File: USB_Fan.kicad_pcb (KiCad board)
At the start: 4 copper layers, 35.1 x 24.9 mm, 38 parts, among them J1 USB-C (Female), J2 Fan, J3 Fan Voltage, SW1 Power, U1 TP4056, U2 DW01A-G, U3 FS8205A, U4 TPS61170

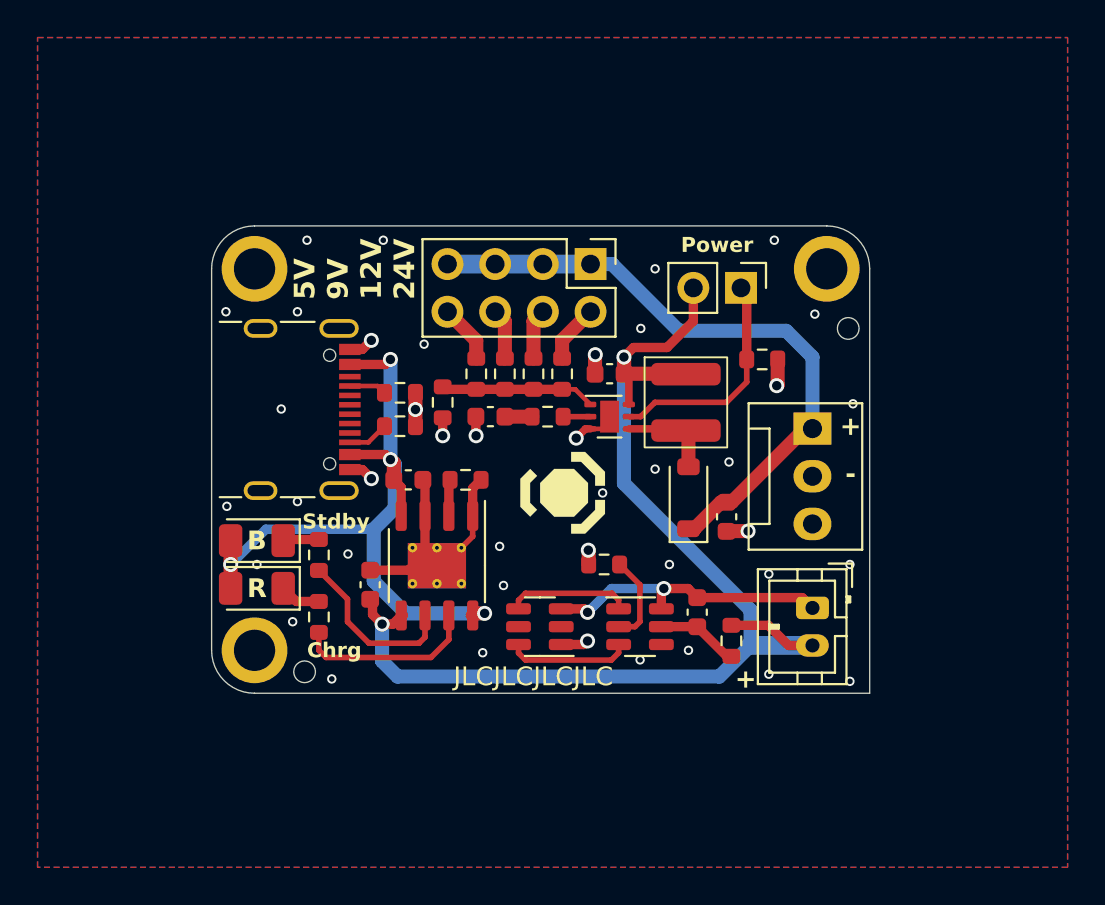
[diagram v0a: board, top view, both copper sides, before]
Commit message: Revision 2
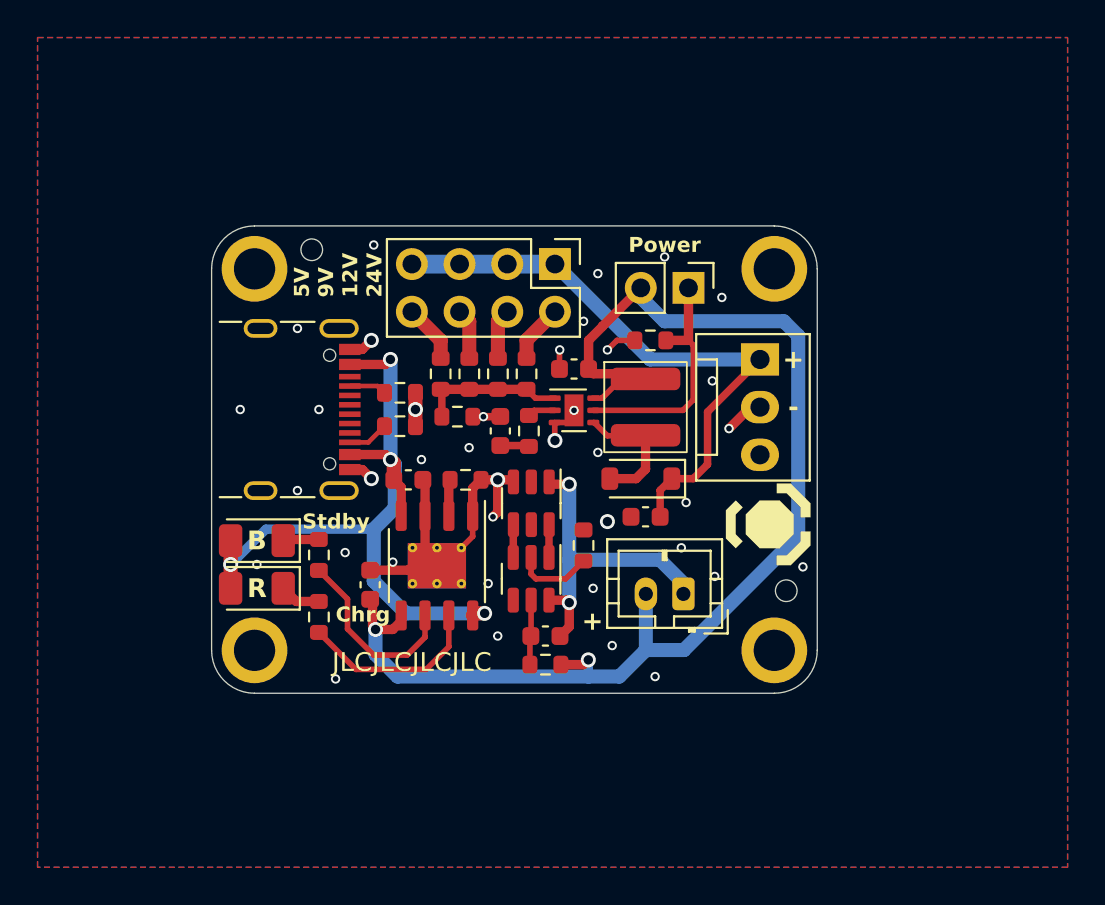
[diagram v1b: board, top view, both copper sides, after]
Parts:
- added H5: MountingHole_Pad, MountingHole:MountingHole_2.2mm_M2_ISO7380_Pad, F.Cu at (108.5, 59.9)
- moved H1 22.5 mm to (83.8, 38.6)
- moved H2 14.4 mm to (109.1, 56.8)
- moved R7 9.99 mm to (96.3, 60.7), turned to 0 degrees
- moved C3 8.19 mm to (96.3, 59.2), turned to 0 degrees
- moved BT1 6.91 mm to (103.6, 56.9), turned to 180 degrees
- moved U3 6.59 mm to (95.5, 52.1), turned to -90 degrees
- moved U2 6.34 mm to (95.5, 56.1), turned to -90 degrees
- moved R14 6.04 mm to (101.9, 43.4), turned to 180 degrees
- moved J2 4.62 mm to (107.7, 44.5)
- moved C6 4.32 mm to (101.6, 52.8), turned to 180 degrees
- moved SW1 2.80 mm to (103.9, 40.6)
- moved H4 2.79 mm to (108.5, 39.6)
- moved D1 2.74 mm to (101.3, 50.8), turned to 180 degrees
- moved L1 2.16 mm to (101.6, 47.0)
- moved U4 1.92 mm to (97.8, 47.2)
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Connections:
- J1 pad S1: unconnected-(J1-SHIELD-PadS1) -> GND
- U3 pad 1: GND -> -BATT
- U3 pad 3: -BATT -> GND
- U3 pad 4: /FET Discharge -> /FET Charge
- U3 pad 6: /FET Charge -> /FET Discharge
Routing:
- net +BATT: track 63.9 -> 68.7 mm
- net /FET Discharge: track 6.56 -> 1.75 mm
- net /FET Charge: track 6.54 -> 1.75 mm
- net /V_{OUT}: track 34.1 -> 31.9 mm
- net -BATT: track 15.6 -> 17.7 mm
- net Net-(D1-A): track 5.06 -> 7.00 mm
- net GND: track 27.3 -> 29.0 mm, vias 41 -> 39
- net /DW01A Vcc: track 4.38 -> 3.46 mm
- net /Standby: track 9.25 -> 10.0 mm
- net Net-(SW1-A): track 12.2 -> 12.8 mm
- net Net-(U2-VM): track 4.74 -> 4.18 mm
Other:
- board size 35.1 x 24.9 mm -> 32.3 x 24.9 mm
- board text removed: "1S LiPo USB-C Multiple voltages"
